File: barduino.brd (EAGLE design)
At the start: 55 x 49.6 mm, 25 parts, among them Q2 16MHz, X1 MINI-USB-UX60A-MB-5ST

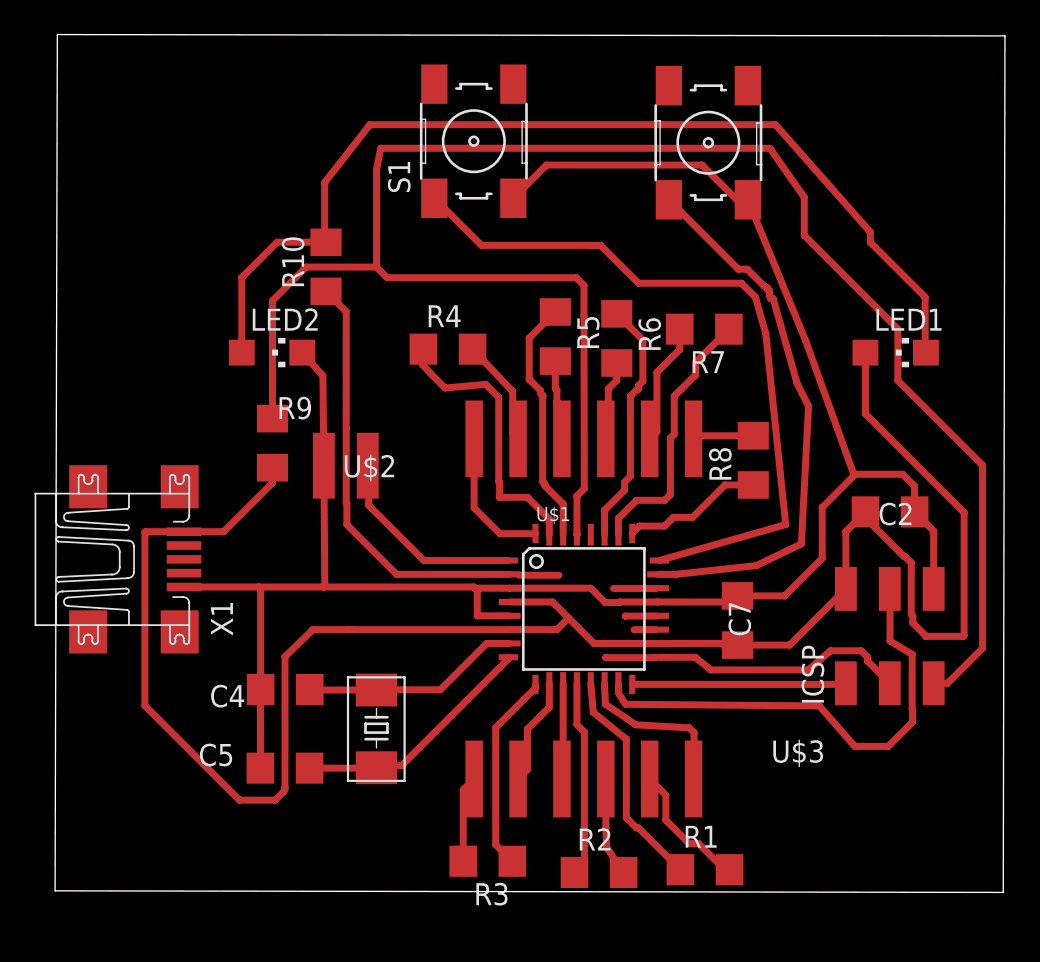
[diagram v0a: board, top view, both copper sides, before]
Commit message: made the routing pretty(ier)
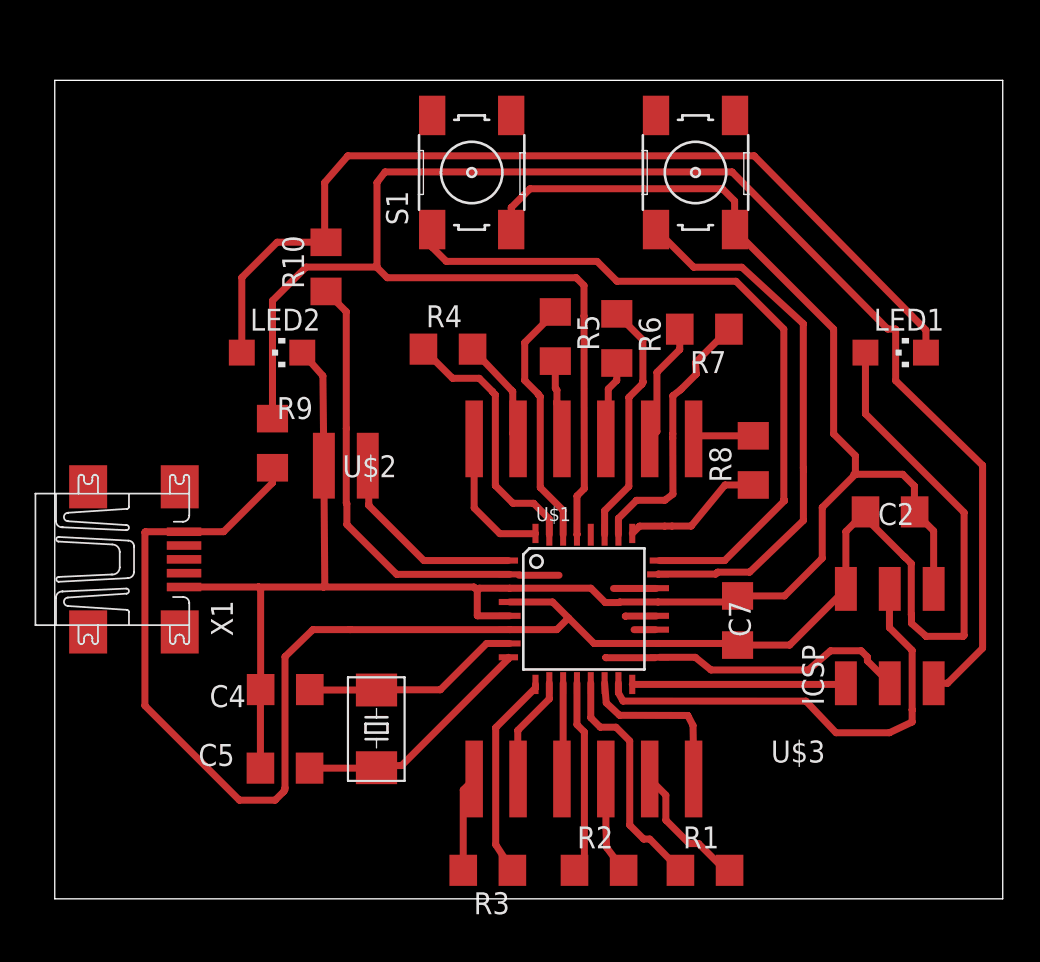
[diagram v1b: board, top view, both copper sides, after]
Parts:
- moved S0 1.88 mm to (17.3, 54.4)
- moved S1 1.82 mm to (4.32, 54.4)
- moved R3 0.52 mm to (5.25, 14.0)
- moved R2 0.13 mm to (11.7, 14.0)
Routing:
- net RESET: track 107.7 -> 104.0 mm
- net N$5: track 57.9 -> 54.7 mm
- net GND: track 114.7 -> 116.3 mm
- net MOSI-D11: track 28.0 -> 27.0 mm
- net D1: track 16.3 -> 15.4 mm
- net D9: track 13.1 -> 13.7 mm
- net N$4: track 5.02 -> 5.55 mm
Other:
- board size 55 x 49.6 mm -> 54.9 x 47.4 mm
